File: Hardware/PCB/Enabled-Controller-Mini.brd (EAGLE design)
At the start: 54 x 39 mm, 10 parts

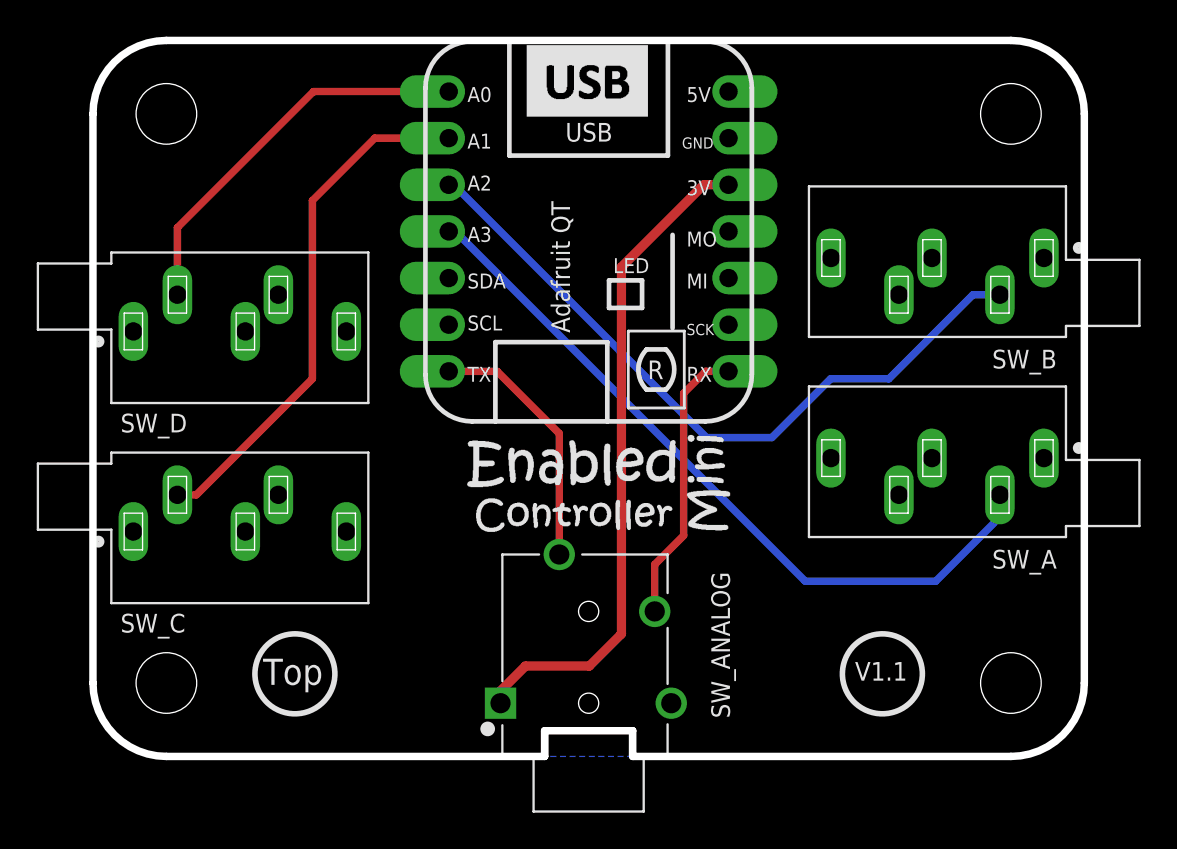
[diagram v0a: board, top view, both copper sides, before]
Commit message: Reversed PCB design file
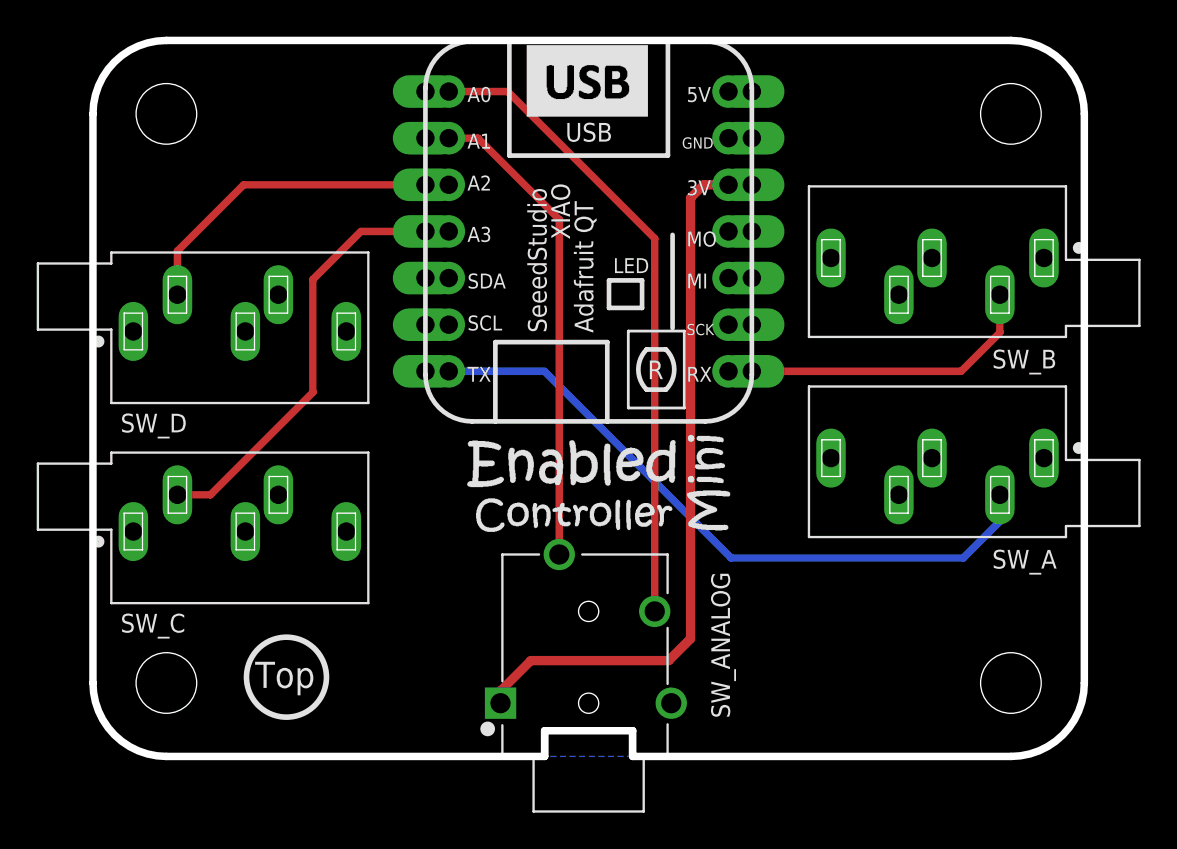
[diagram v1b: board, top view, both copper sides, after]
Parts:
- U$1: value ADAFRUIT_QT_PY -> SEEEDSTUDIO_XIAO_QT; device MMC Eagle:QT_PY -> MMC Eagle:SEEEDSTUDIO_XIAO
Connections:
- removed net N$3: SW_D.2, U$1.A0
- new net N$11: SW_D.2, U$1.A2_0, U$1.A2_1
- net +3V3: now also U$1.3V_0, U$1.3V_1; no longer U$1.3V
- net GND: now also U$1.GND_0, U$1.GND_1; no longer U$1.GND
- net N$1: now also U$1.RX_0, U$1.RX_1; no longer U$1.A2
- net N$2: now also U$1.TX_0, U$1.TX_1; no longer U$1.A3
- net N$4: now also U$1.A0_0, U$1.A0_1; no longer U$1.RX
- net N$5: now also U$1.A3_0, U$1.A3_1; no longer U$1.A1
- net N$8: now also U$1.A1_0, U$1.A1_1; no longer U$1.TX
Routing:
- net N$3: track 21.5 -> 0.00 mm
- net N$1: track 38.9 -> 17.7 mm
- net N$4: track 15.5 -> 36.1 mm
- net N$11: track 0.00 -> 18.7 mm
- net N$8: track 14.0 -> 27.4 mm
- net N$5: track 28.5 -> 24.3 mm
- net +3V3: track 36.2 -> 39.8 mm
- net N$2: track 40.6 -> 37.8 mm
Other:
- board text removed: "V1.1"

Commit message: Updated PCB design files : SWITCH GPIO's changed to A0,A1,A2,A3
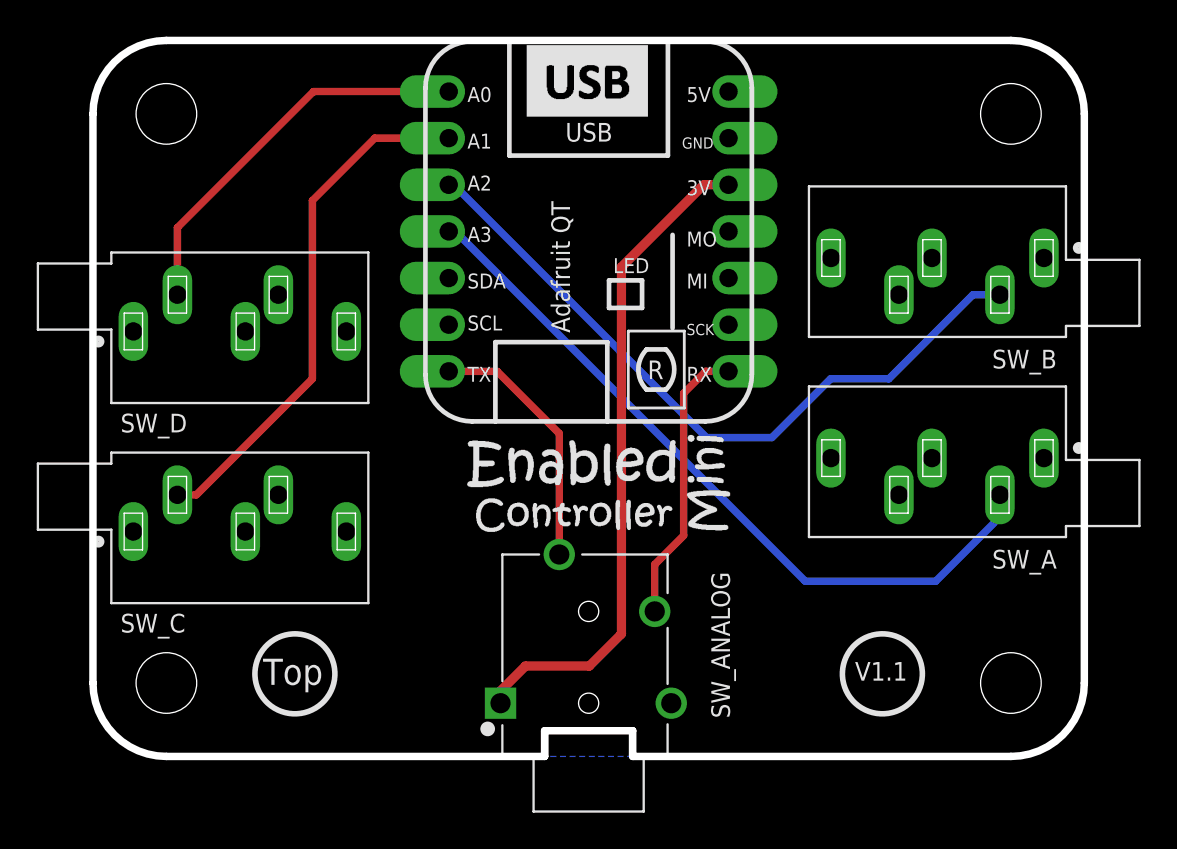
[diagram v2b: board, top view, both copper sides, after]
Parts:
- U$1: value SEEEDSTUDIO_XIAO_QT -> ADAFRUIT_QT_PY; device MMC Eagle:SEEEDSTUDIO_XIAO -> MMC Eagle:QT_PY
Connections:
- removed net N$11: SW_D.2, U$1.A2_0, U$1.A2_1
- new net N$3: SW_D.2, U$1.A0
- net +3V3: now also U$1.3V; no longer U$1.3V_0, U$1.3V_1
- net GND: now also U$1.GND; no longer U$1.GND_0, U$1.GND_1
- net N$1: now also U$1.A2; no longer U$1.RX_0, U$1.RX_1
- net N$2: now also U$1.A3; no longer U$1.TX_0, U$1.TX_1
- net N$4: now also U$1.RX; no longer U$1.A0_0, U$1.A0_1
- net N$5: now also U$1.A1; no longer U$1.A3_0, U$1.A3_1
- net N$8: now also U$1.TX; no longer U$1.A1_0, U$1.A1_1
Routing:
- net N$3: track 0.00 -> 21.5 mm
- net N$1: track 17.7 -> 38.9 mm
- net N$4: track 36.1 -> 15.5 mm
- net N$11: track 18.7 -> 0.00 mm
- net N$8: track 27.4 -> 14.0 mm
- net N$5: track 24.3 -> 28.5 mm
- net +3V3: track 39.8 -> 36.2 mm
- net N$2: track 37.8 -> 40.6 mm
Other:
- board text added: "V1.1"
